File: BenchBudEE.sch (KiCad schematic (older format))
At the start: 0 parts

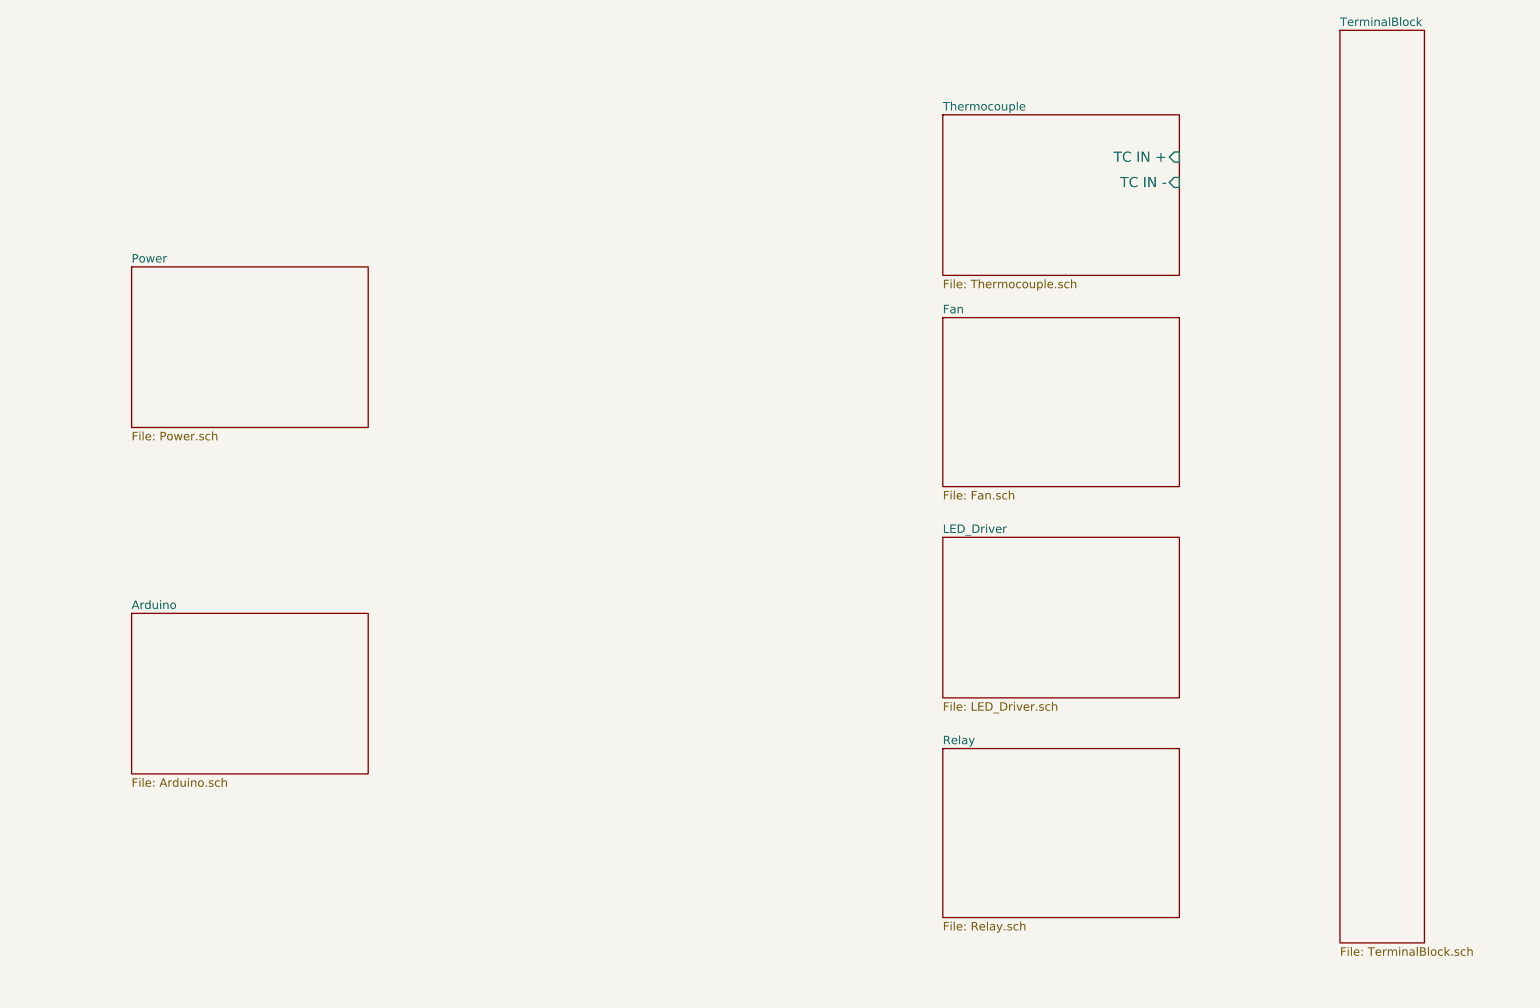
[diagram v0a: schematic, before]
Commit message: Completed -Defining IO Video
http://contextualelectronics.com/module-2/defining-your-inputs-and-outputs/
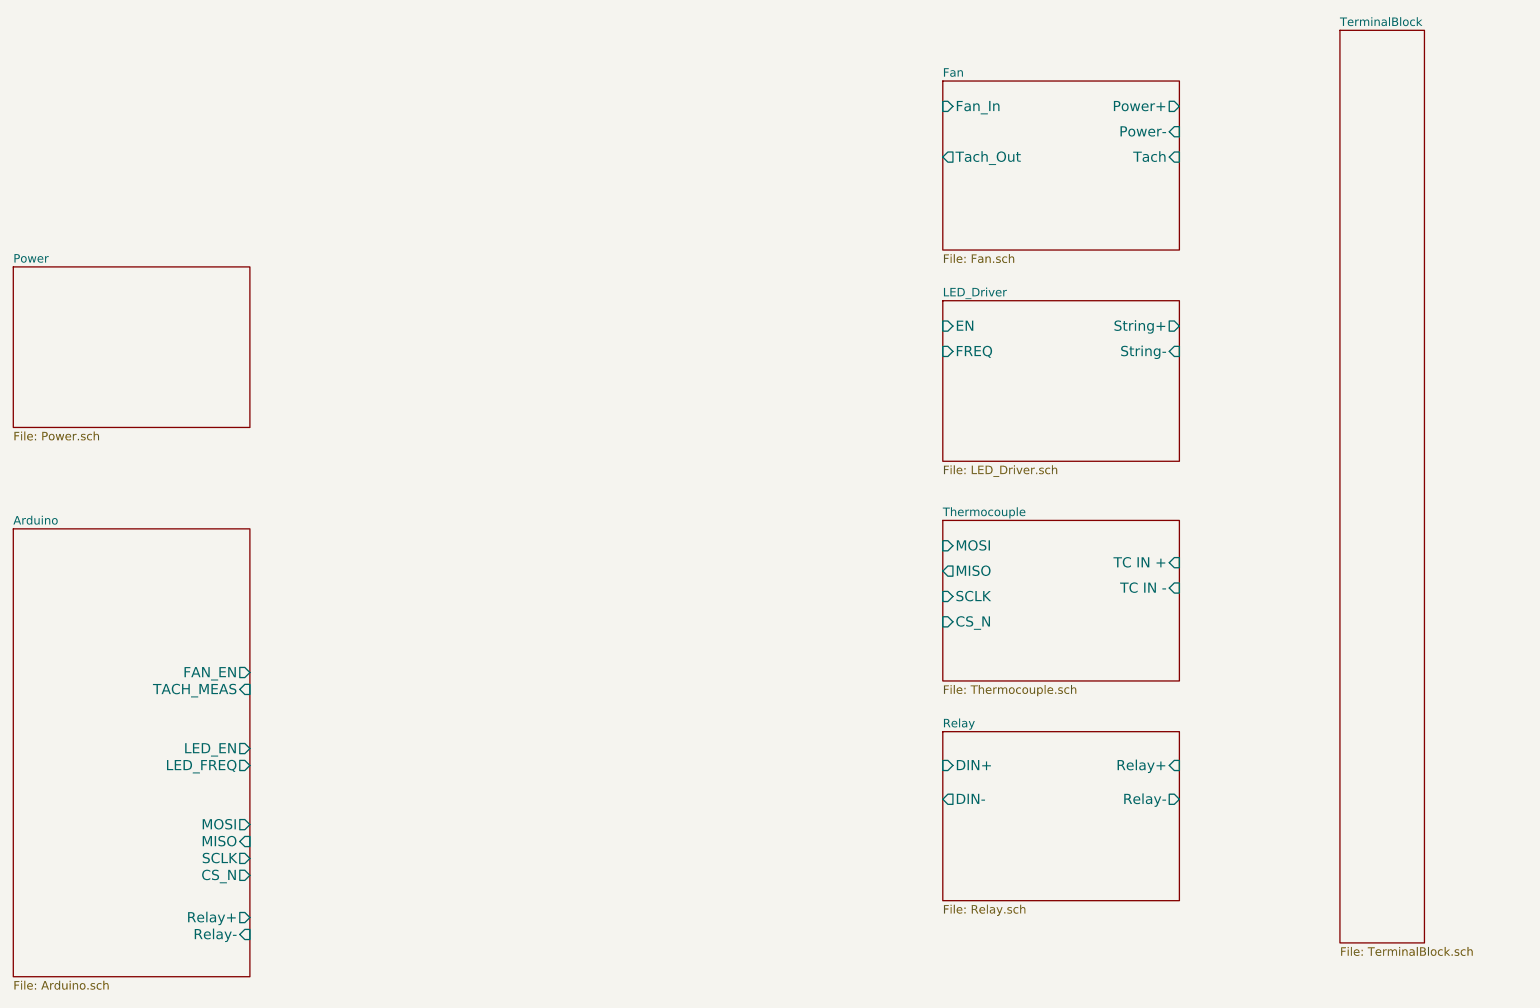
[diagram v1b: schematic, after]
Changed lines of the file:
@@
 $EndDescr
 $Sheet
-S 3200 4900 1400 950
+S 2500 4400 1400 2650
 U 52EEE583
 F0 "Arduino" 50
 F1 "Arduino.sch" 50
+F2 "Relay+" O R 3900 6700 60
+F3 "Relay-" I R 3900 6800 60
+F4 "MOSI" O R 3900 6150 60
+F5 "MISO" I R 3900 6250 60
+F6 "SCLK" O R 3900 6350 60
+F7 "CS_N" O R 3900 6450 60
+F8 "LED_EN" O R 3900 5700 60
+F9 "LED_FREQ" O R 3900 5800 60
+F10 "FAN_EN" O R 3900 5250 60
+F11 "TACH_MEAS" I R 3900 5350 60
 $EndSheet
 $Sheet
-S 8000 1950 1400 950
+S 8000 4350 1400 950
 U 52EEE626
 F0 "Thermocouple" 50
 F1 "Thermocouple.sch" 50
-F2 "TC IN +" I R 9400 2200 60
-F3 "TC IN -" I R 9400 2350 60
+F2 "TC IN +" I R 9400 4600 60
+F3 "TC IN -" I R 9400 4750 60
+F4 "MOSI" I L 8000 4500 60
+F5 "MISO" O L 8000 4650 60
+F6 "SCLK" I L 8000 4800 60
+F7 "CS_N" I L 8000 4950 60
 $EndSheet
 $Sheet
-S 8000 5700 1400 1000
+S 8000 5600 1400 1000
 U 52EEE642
 F0 "Relay" 50
 F1 "Relay.sch" 50
+F2 "DIN+" I L 8000 5800 60
+F3 "DIN-" O L 8000 6000 60
+F4 "Relay+" I R 9400 5800 60
+F5 "Relay-" O R 9400 6000 60
 $EndSheet
 $Sheet
-S 3200 2850 1400 950
+S 2500 2850 1400 950
 U 52EEE692
 F0 "Power" 50
@@
 $EndSheet
 $Sheet
-S 8000 4450 1400 950
+S 8000 3050 1400 950
 U 52EEE6FA
 F0 "LED_Driver" 50
 F1 "LED_Driver.sch" 50
+F2 "EN" I L 8000 3200 60
+F3 "FREQ" I L 8000 3350 60
+F4 "String+" O R 9400 3200 60
+F5 "String-" I R 9400 3350 60
 $EndSheet
 $Sheet
-S 8000 3150 1400 1000
+S 8000 1750 1400 1000
 U 52EEE752
 F0 "Fan" 50
 F1 "Fan.sch" 50
+F2 "Power+" O R 9400 1900 60
+F3 "Power-" I R 9400 2050 60
+F4 "Tach" I R 9400 2200 60
+F5 "Tach_Out" O L 8000 2200 60
+F6 "Fan_In" I L 8000 1900 60
 $EndSheet
 $Sheet
